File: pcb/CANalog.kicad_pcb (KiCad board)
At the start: 2 copper layers, 100 x 45 mm, 96 parts, among them J1 PWR, J2 USB_B_Micro, J3 SPI3, J4 I2C2, J5 STM_PROG, J6 ESP_PROG, J7 AOUT, J8 CAN, Q1 DMP3099L-7, Q2 MMBT2222A, Q3 DMP3099L-7, SW1 RESET, SW2 ESP_PROG, U1 BL9342, U2 RS321BXF, U3 STM32F302C8T6, U4 ESP-12F, U5 MIC5504-3.3YM5, U6 OPA330xxDBV, U7 SN65HVD230, U8 74AHC1G66, Y1 16MHz

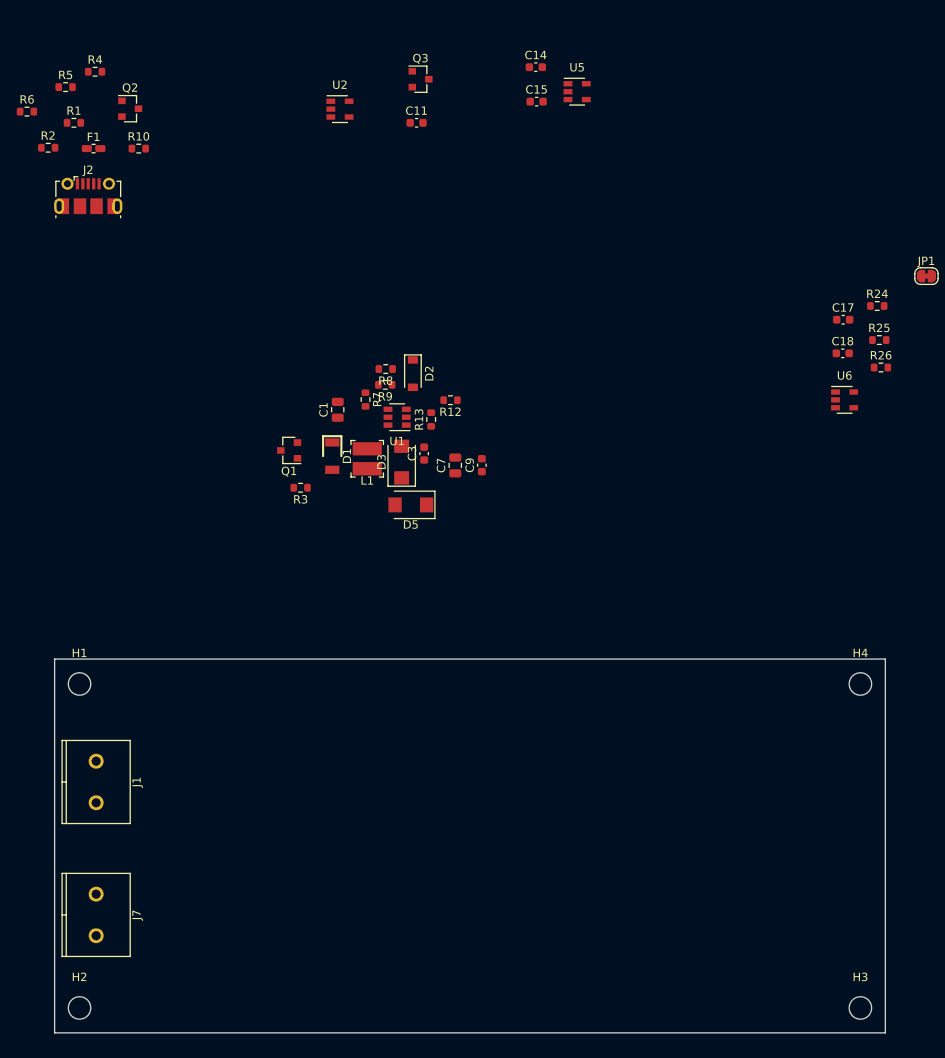
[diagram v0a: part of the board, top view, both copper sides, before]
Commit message: Update CANalog.kicad_pcb
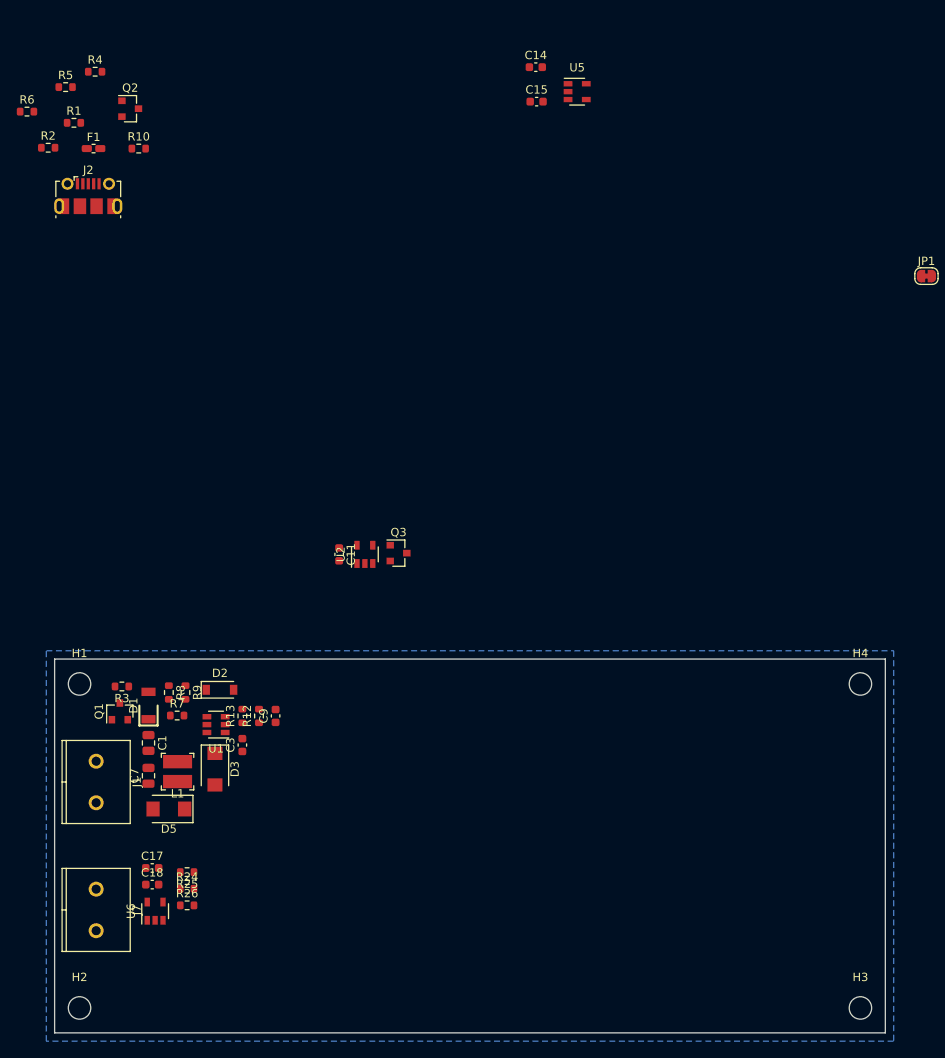
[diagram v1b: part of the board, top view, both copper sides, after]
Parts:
- moved R24 108.7 mm to (41.0, 167.7)
- moved C17 106.2 mm to (36.8, 165.2)
- moved R26 105.7 mm to (41.0, 169.7)
- moved R25 105.1 mm to (41.0, 165.7), turned to 180 degrees
- moved C18 104.9 mm to (36.8, 167.2)
- moved U6 103.3 mm to (37.1, 170.3), turned to 90 degrees
- moved Q3 57.1 mm to (66.4, 127.2)
- moved U2 53.7 mm to (62.4, 127.4), turned to 90 degrees
- moved C11 52.8 mm to (59.2, 127.4), turned to 270 degrees
- moved C7 52.5 mm to (36.3, 154.1)
- moved R8 46.9 mm to (38.8, 144.0), turned to 270 degrees
- moved D5 46.8 mm to (38.8, 158.1)
- moved C1 46.1 mm to (36.3, 150.1), turned to 270 degrees
- moved D2 44.6 mm to (44.9, 143.7), turned to 0 degrees
- moved R12 44.5 mm to (49.6, 146.8), turned to 90 degrees
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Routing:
- added copper zone on B.Cu, net GND
